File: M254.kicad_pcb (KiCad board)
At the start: 2 copper layers, 12 parts, among them J1 from Sensor, J2 to M304, U1 NJM2903

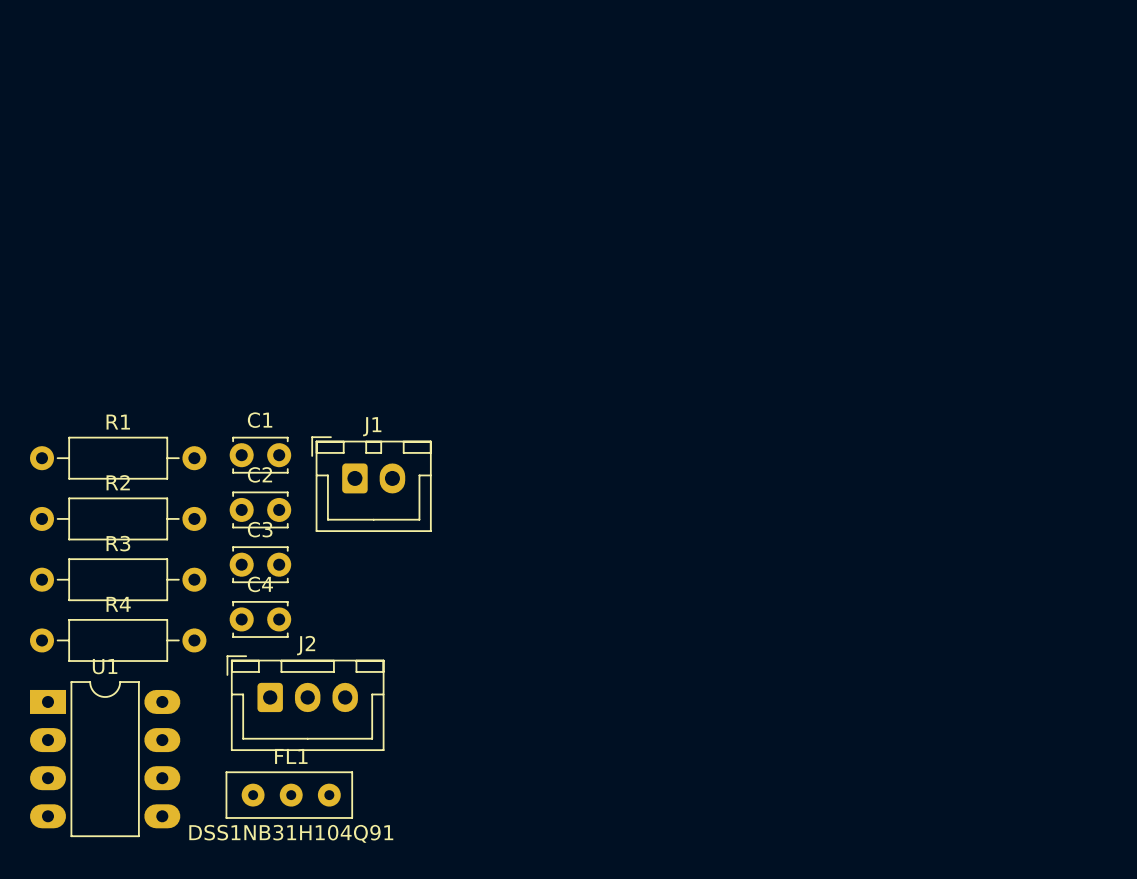
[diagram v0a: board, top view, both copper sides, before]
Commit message: 途中
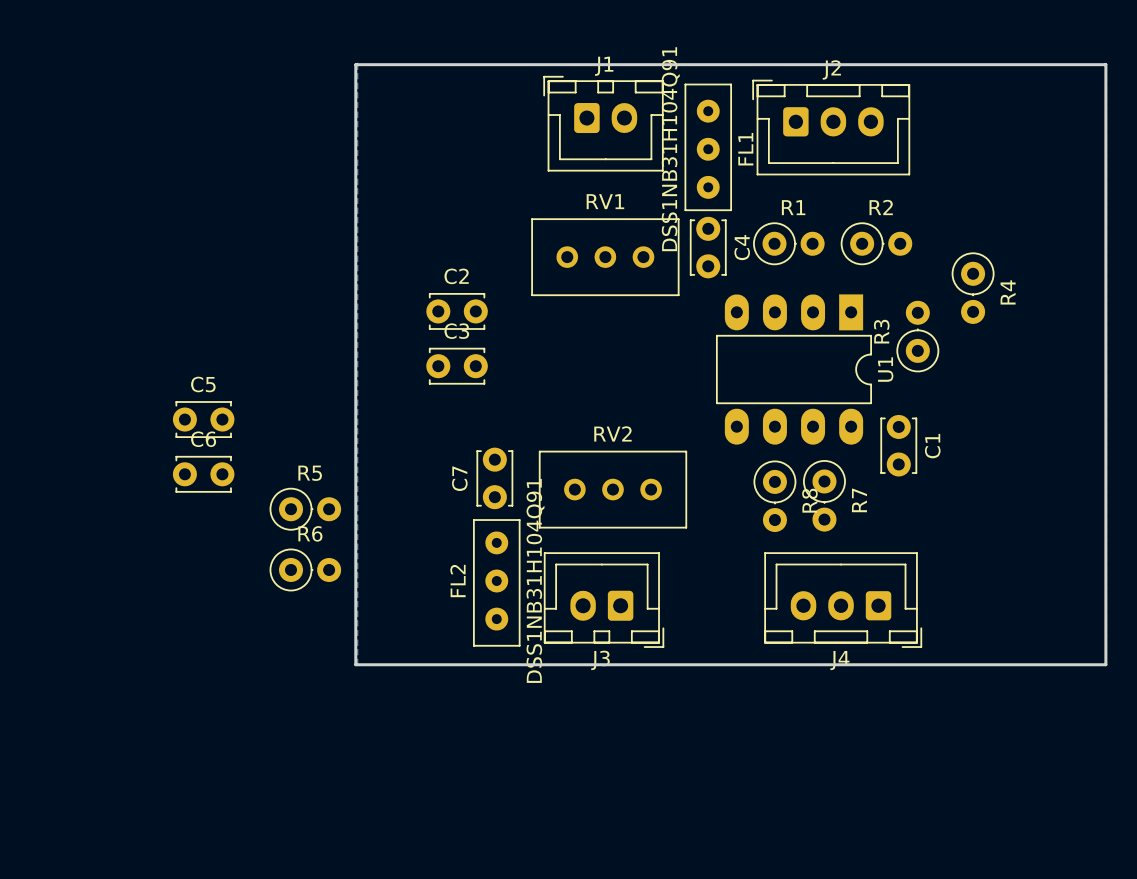
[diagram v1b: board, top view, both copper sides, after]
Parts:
- added C5: 0.1uF, Capacitor_THT:C_Disc_D3.4mm_W2.1mm_P2.50mm, F.Cu at (124.4, 91.0)
- added C6: 0.1uF, Capacitor_THT:C_Disc_D3.4mm_W2.1mm_P2.50mm, F.Cu at (124.4, 94.6)
- added C7: 0.1uF, Capacitor_THT:C_Disc_D3.4mm_W2.1mm_P2.50mm, F.Cu at (145.0, 96.1)
- added FL2: DSS1NB31H104Q91, HOLLY2:DSS1, F.Cu at (145.2, 101.7)
- added J3: from Sensor2, Connector_JST:JST_XH_B2B-XH-A_1x02_P2.50mm_Vertical, F.Cu at (153.4, 103.4)
- added J4: to M304, Connector_JST:JST_XH_B3B-XH-A_1x03_P2.50mm_Vertical, F.Cu at (170.6, 103.4)
- added R5: 47k, Resistor_THT:R_Axial_DIN0207_L6.3mm_D2.5mm_P2.54mm_Vertical, F.Cu at (131.4, 96.9)
- added R6: 2k, Resistor_THT:R_Axial_DIN0207_L6.3mm_D2.5mm_P2.54mm_Vertical, F.Cu at (131.4, 101.0)
- added R7: 10k, Resistor_THT:R_Axial_DIN0207_L6.3mm_D2.5mm_P2.54mm_Vertical, F.Cu at (167.0, 95.1)
- added R8: 1M, Resistor_THT:R_Axial_DIN0207_L6.3mm_D2.5mm_P2.54mm_Vertical, F.Cu at (163.7, 95.1)
- added RV1: 50k, Potentiometer_THT:Potentiometer_Bourns_3296W_Vertical, F.Cu at (154.9, 80.1)
- added RV2: 50k, Potentiometer_THT:Potentiometer_Bourns_3296W_Vertical, F.Cu at (155.4, 95.6)
- FL1: footprint holly:DSS1 -> HOLLY2:DSS1
- J1: value from Sensor -> from Sensor1
- R1, R2, R3, R4: footprint Resistor_THT:R_Axial_DIN0207_L6.3mm_D2.5mm_P10.16mm_Horizontal -> Resistor_THT:R_Axial_DIN0207_L6.3mm_D2.5mm_P2.54mm_Vertical
- moved R4 66.7 mm to (176.9, 81.3), turned to -90 degrees
- moved R3 60.3 mm to (173.2, 86.4), turned to 90 degrees
- moved U1 59.5 mm to (168.8, 83.8), turned to -90 degrees
- moved R2 57.7 mm to (169.5, 79.2)
- moved J2 52.0 mm to (165.1, 71.1)
- moved FL1 51.2 mm to (159.3, 72.9), turned to -90 degrees
- moved R1 50.9 mm to (163.7, 79.2)
- moved C1 43.8 mm to (172.0, 91.5), turned to -90 degrees
- moved C4 40.6 mm to (159.3, 78.3), turned to -90 degrees
- moved J1 28.6 mm to (151.2, 70.9)
- moved C2 18.6 mm to (141.3, 83.8)
- moved C3 18.6 mm to (141.3, 87.4)
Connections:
- U1 pad 5: unconnected-(U1B-+-Pad5) -> Net-(U1B-+)
- U1 pad 6: unconnected-(U1B---Pad6) -> Net-(U1B--)
- U1 pad 7: unconnected-(U1-Pad7) -> Net-(J4-Pin_2)
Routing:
- added copper zone on B.Cu, net GND
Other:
- board outline added: 50 x 40 mm
